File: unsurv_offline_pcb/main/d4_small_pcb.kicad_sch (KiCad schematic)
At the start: 54 parts, among them J1 U_FL-R-SMT-1_10_, J2 S2B-PH-SM4-TB_LF__SN_, Q1 UMH3N, Q2 Q_PMOS_GSD, U1 TTGO-Micro32-ESP32, U2 MCP73831-2-OT, U3 CAM-M8C-0-10, U4 AP2112K-3.3, U5 CH340G, U6 RF430CL330H, U7 BMA400-I2C, U8 RFM95W-868S2

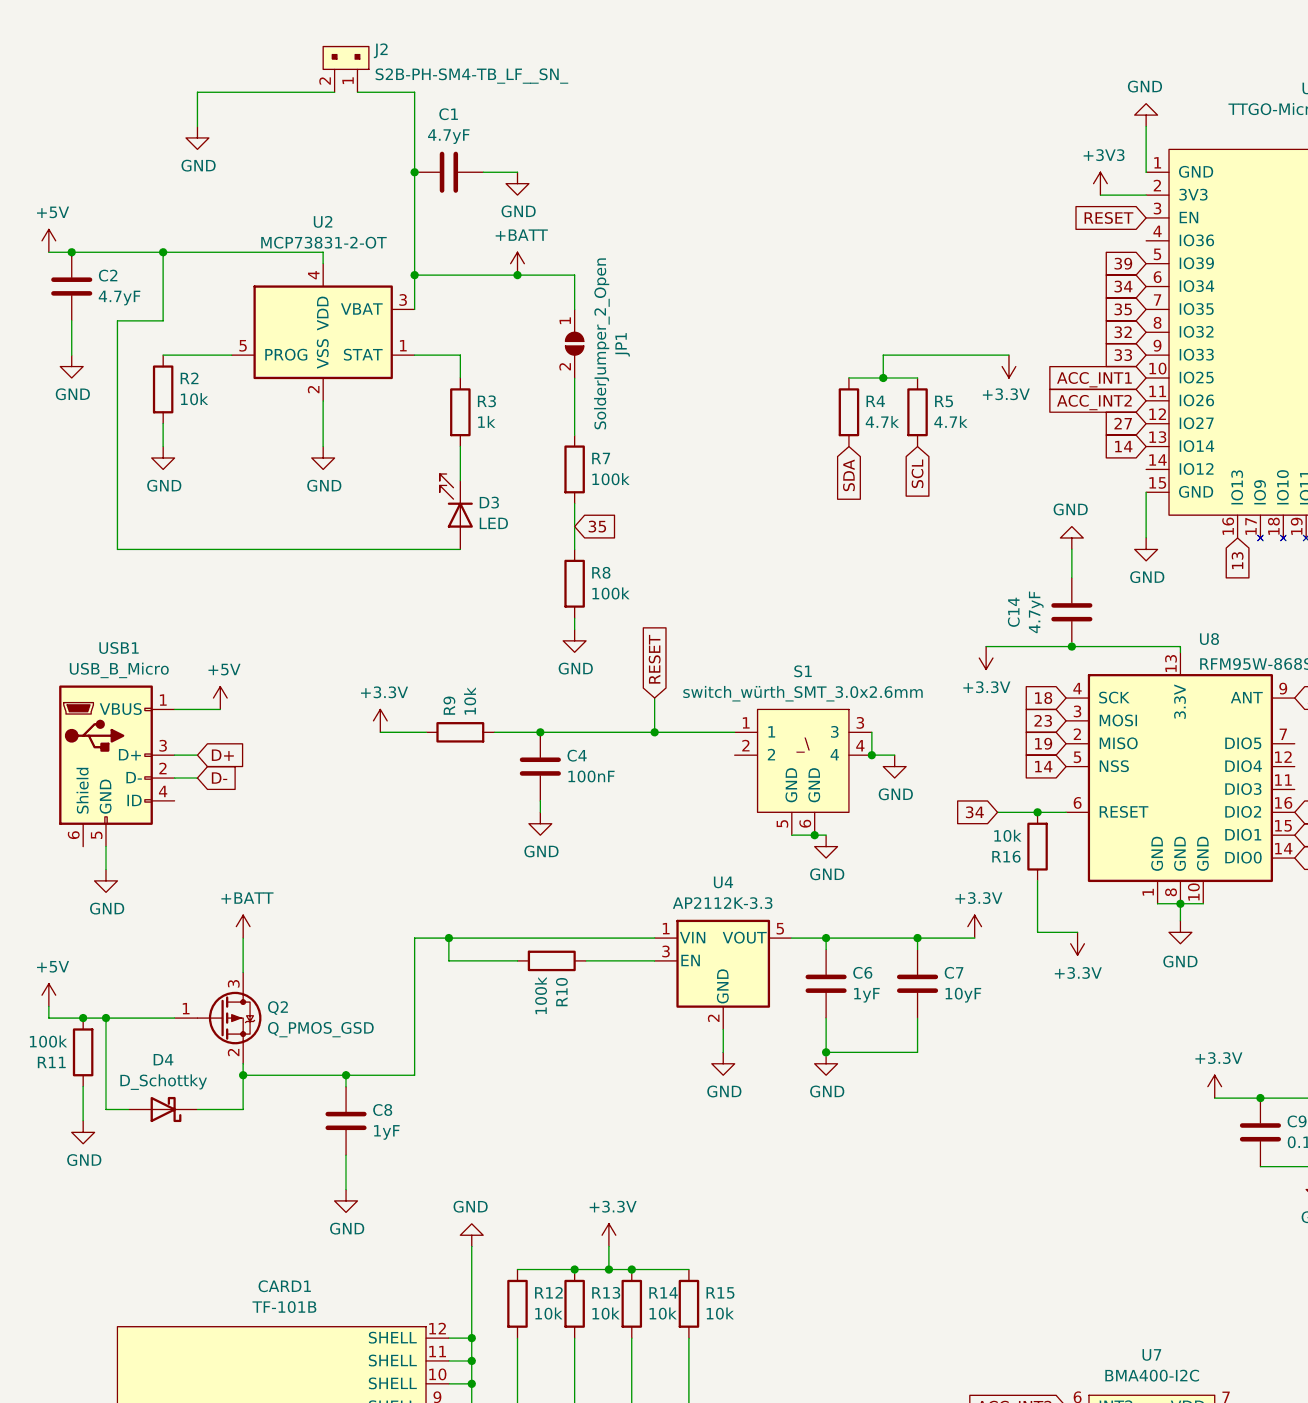
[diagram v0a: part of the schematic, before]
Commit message: pre rework
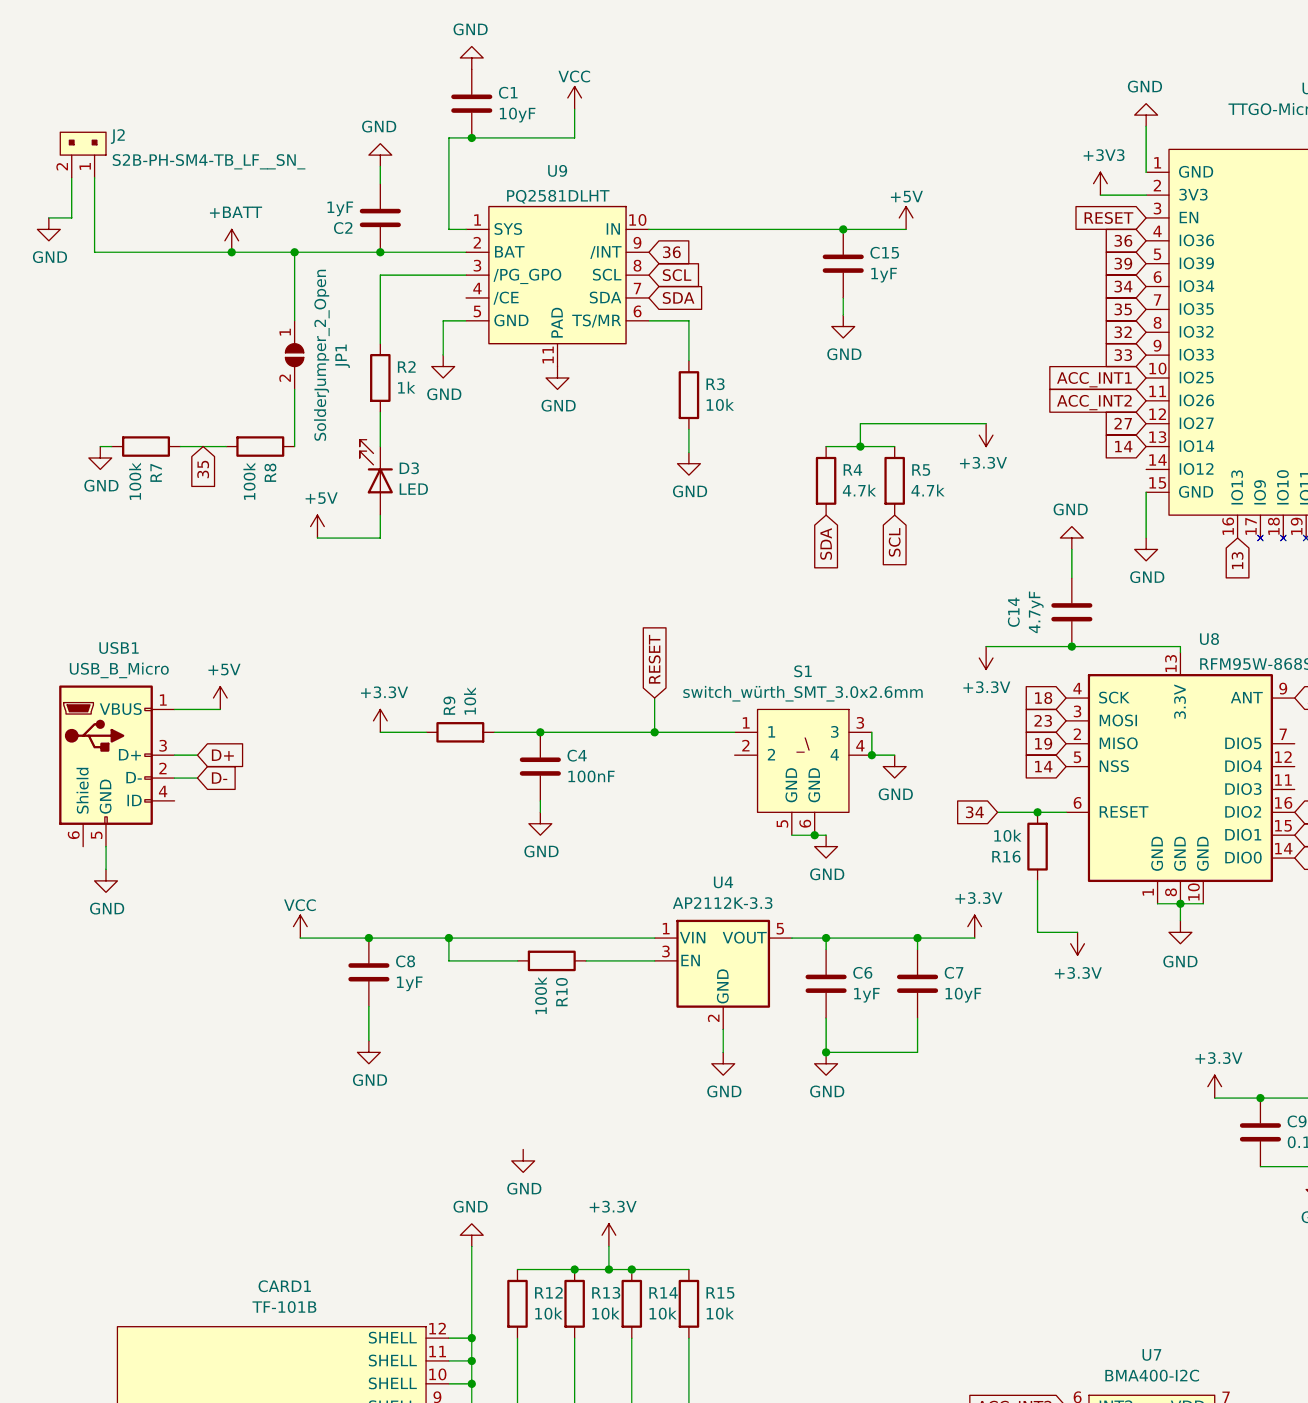
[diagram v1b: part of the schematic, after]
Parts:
- removed D4: D_Schottky, Diode_SMD:D_SOD-323, symbol Device:D_Schottky
- removed Q2: Q_PMOS_GSD, Package_TO_SOT_SMD:SOT-23, symbol Device:Q_PMOS_GSD
- removed R11: 100k, Resistor_SMD:R_0603_1608Metric, symbol Device:R
- removed U2: MCP73831-2-OT, Package_TO_SOT_SMD:SOT-23-5, symbol Battery_Management:MCP73831-2-OT
- added C15: 1yF, Capacitor_SMD:C_0603_1608Metric, symbol Device:C
- added U9: PQ2581DLHT, unsurv_offline_pcb_footprints:BQ2581DLHT, symbol unsurv_offline_pcb_symbols:PQ2581DLHT
- C1: value 4.7yF -> 10yF
- C2: value 4.7yF -> 1yF
- R2: value 10k -> 1k
- R3: value 1k -> 10k
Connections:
- net +5V: now also C15.2, U9.10 (IN); no longer C2.2
- net +BATT: now also C2.2, U9.2 (BAT); no longer C1.2
- net 35: now also R7.1, R8.2; no longer R7.2, R8.1
- net GND: now also C1.2, R3.2, R7.2, C15.1, U9.11 (PAD), U9.5 (GND); no longer C1.1, R2.2, R8.2
- net SCL: now also U9.8 (SCL)
- net SDA: now also U9.7 (SDA)
- net at R3.1: now also U9.6 (TS/MR)
- net at R2.1: now also U9.3 (/PG_GPO)
- net at D3.1 (K): now also R2.2; no longer R3.2
- net VCC: now reaches C8.2, R10.2, U4.1 (VIN)
- net VCC: now also C1.1, U9.1 (SYS)
- net at JP1.2 (B): now also R8.1; no longer R7.1
- net 36: now reaches U1.4 (IO36)
- net 36: now also U9.9 (/INT)
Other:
- moved on the sheet: C8, J2, R4, R5
